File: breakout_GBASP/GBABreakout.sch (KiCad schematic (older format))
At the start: 17 parts, among them J1 Conn_01x16, J10 TP8, J11 TP3, J12 TP2, J13 S02, J14 S01, J15 CK1, J16 BAT+, J17 GND, J2 VCC, J3 TP6, J4 TP7, J5 TP5, J6 TP4, J7 TP0, J8 TP1, J9 TP9

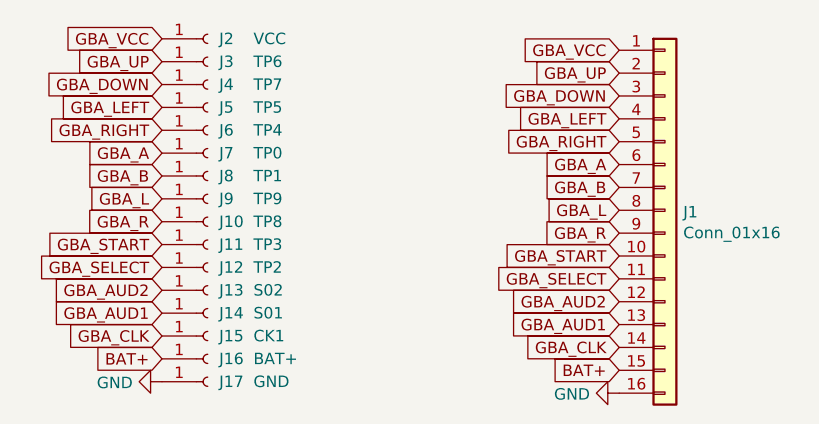
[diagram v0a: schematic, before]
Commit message: updated shield
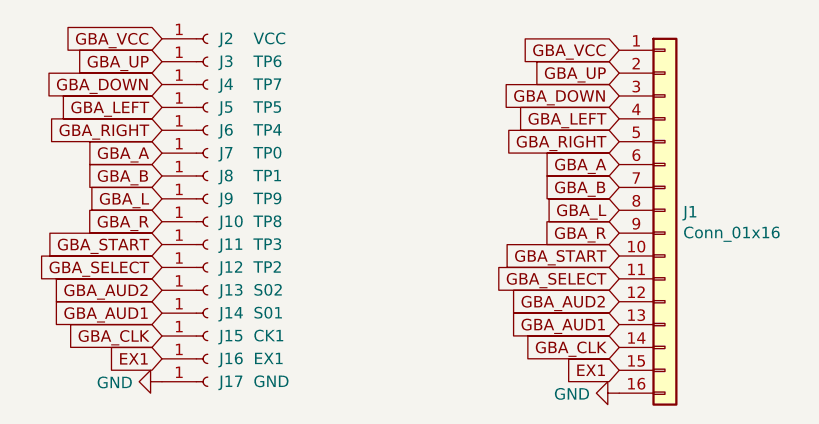
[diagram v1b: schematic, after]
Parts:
- J16: value BAT+ -> EX1
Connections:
- net BAT+ renamed EX1
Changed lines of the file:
@@
 GBA_L
 Text GLabel 4800 2850 0    50   Input ~ 0
-BAT+
+EX1
 Text GLabel 2800 2800 0    50   Input ~ 0
-BAT+
+EX1
 $Comp
 L power:GND #PWR0102
@@
 P 3000 2800
 F 0 "J16" H 3050 2800 50  0000 L CNN
-F 1 "BAT+" H 3200 2800 50  0000 L CNN
+F 1 "EX1" H 3200 2800 50  0000 L CNN
 F 2 "OFFSET:SOLDER_PAD" H 3000 2800 50  0001 C CNN
 F 3 "~" H 3000 2800 50  0001 C CNN
